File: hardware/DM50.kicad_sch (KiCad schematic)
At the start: 99 parts, among them J1 ST-LINK, J2 USB_C_Receptacle_USB2.0_14P, Q1 MMBT3904, SW10 CST, SW11 VAR, SW12 U, SW13 NXT, SW14 quote, SW15 STO, SW16 EVAL, SW17 L, SW18 D, SW19 R, SW2 F1, SW20 SIN, SW21 COS, SW22 TAN, SW23 SQR, SW24 y^x, SW25 1/x, SW26 ENTER, SW27 ENTER, SW28 +/-, SW29 EEX, SW3 F2, SW30 DEL, SW31 BACK, SW32 ALPHA, SW33 7, SW34 8, SW35 9, SW36 /, SW37 OPT1, SW38 4, SW39 5, SW4 F3, SW40 6, SW41 x, SW42 RESET, SW43 OPT2, SW44 1, SW45 2, SW46 3, SW47 -, SW48 ON, SW49 0, SW5 F4, SW50 ., SW51 SPC, SW52 +, SW6 F5, SW7 F6, SW8 MTH, SW9 PRG, U1 EA_DOGL128X-6, U2 STM32U535CBT6, U3 AT25SF641, U4 USBLC6-2SC6, U5 ADP2108AUJ-3.3, Y1 32768

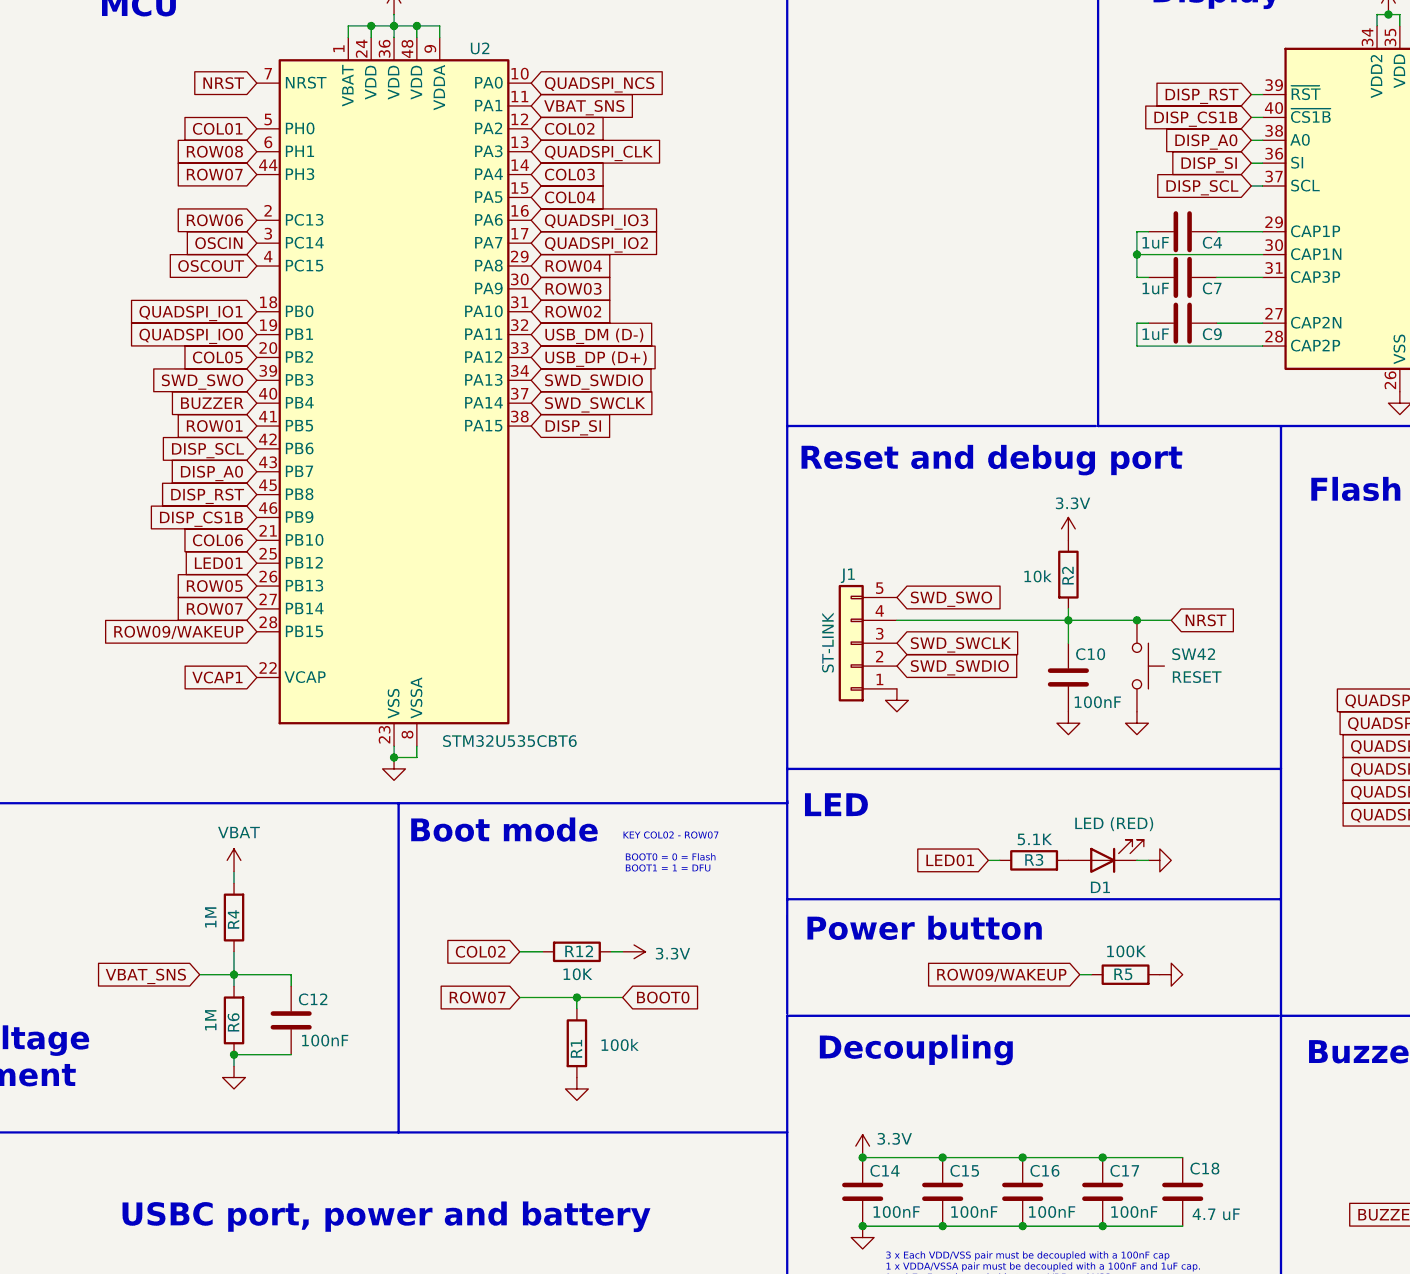
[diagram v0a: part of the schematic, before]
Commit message: pcb changes
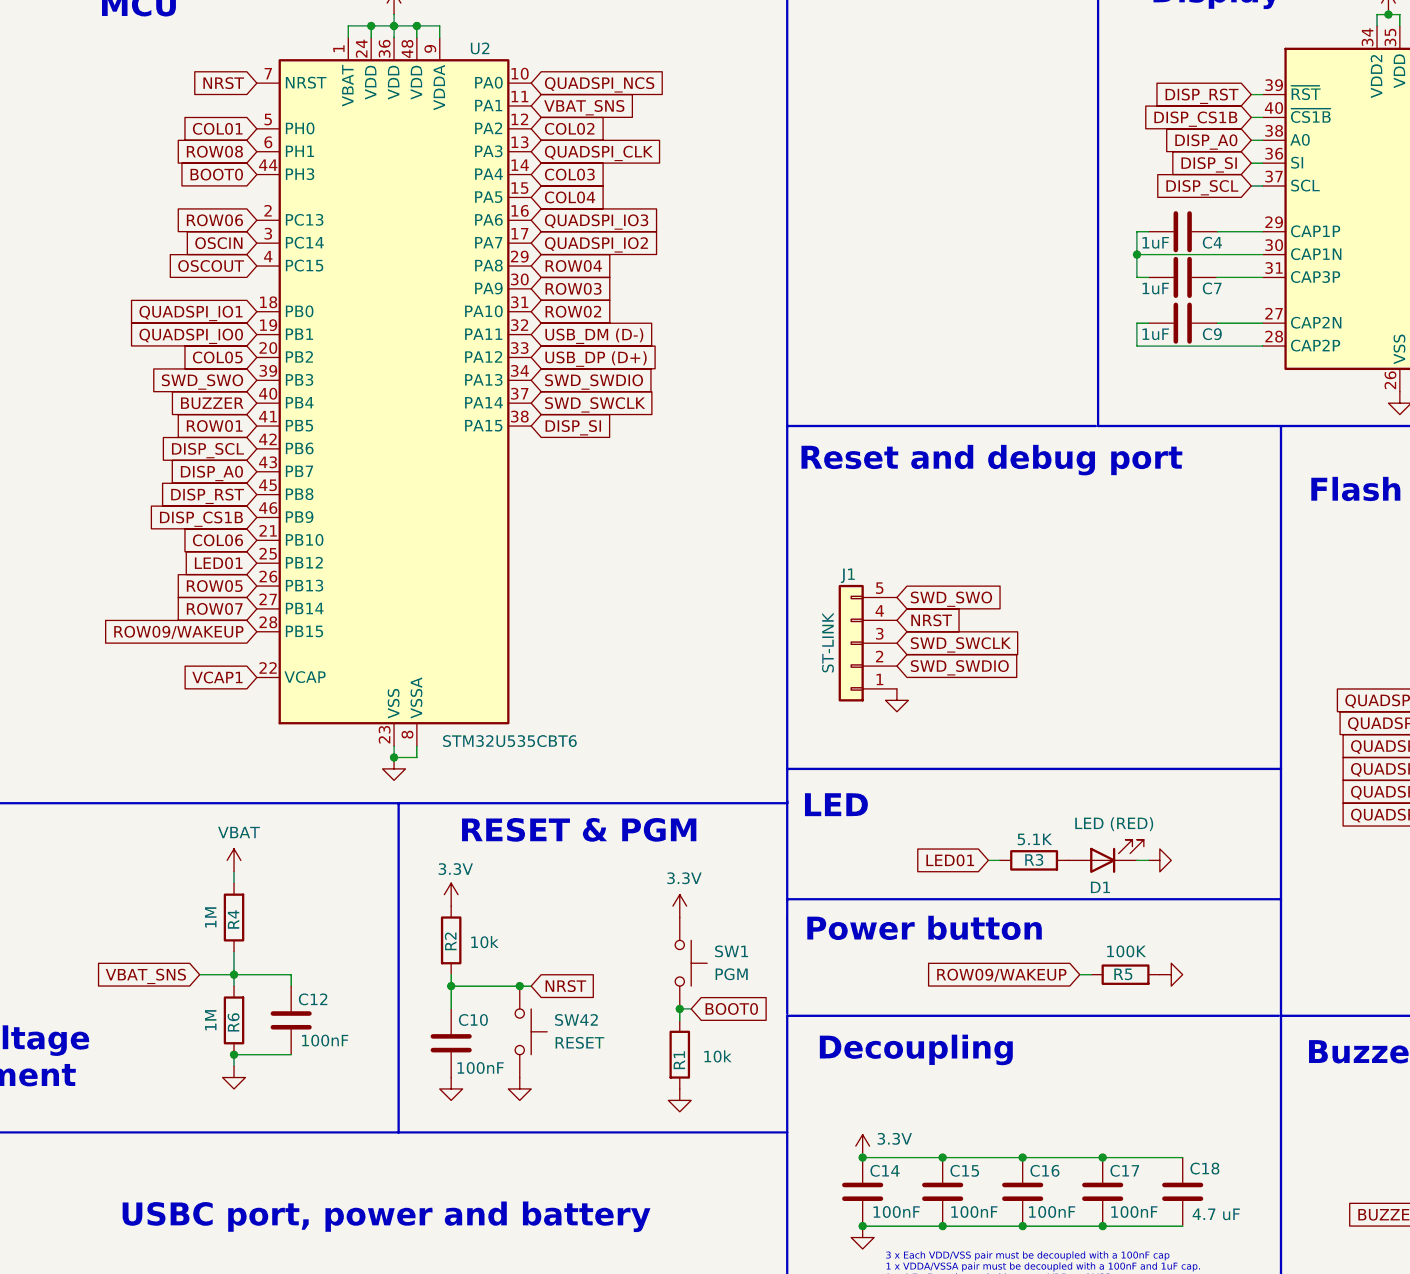
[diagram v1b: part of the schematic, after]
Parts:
- removed R12: 10K, Resistor_SMD:R_0603_1608Metric, symbol Device:R
- added SW1: PGM, Button_Switch_SMD:SW_SPST_TL3342, symbol Switch:SW_Push
- R1: value 100k -> 10k
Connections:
- net 3.3V: now also SW1.1
- net BOOT0: now also SW1.2; no longer SW37.2, SW38.2, SW39.2, SW40.2, SW41.2, U2.27 (PB14)
- new net ROW07: SW37.2, SW38.2, SW39.2, SW40.2, SW41.2, U2.27 (PB14)
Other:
- note added: "RESET & PGM"
- note removed: "BOOT0 = 0 = Flash BOOT1 = 1 = DFU"
- note removed: "Boot mode"
- note removed: "KEY COL02 - ROW07"
- moved on the sheet: C10, R1, R2, SW42
